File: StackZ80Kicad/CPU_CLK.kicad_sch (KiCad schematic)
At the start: 13 parts, among them SW4 SW_Push, U3 Z84C0008P, U6 74HCT04, Y1 7.3728MHz Crystal

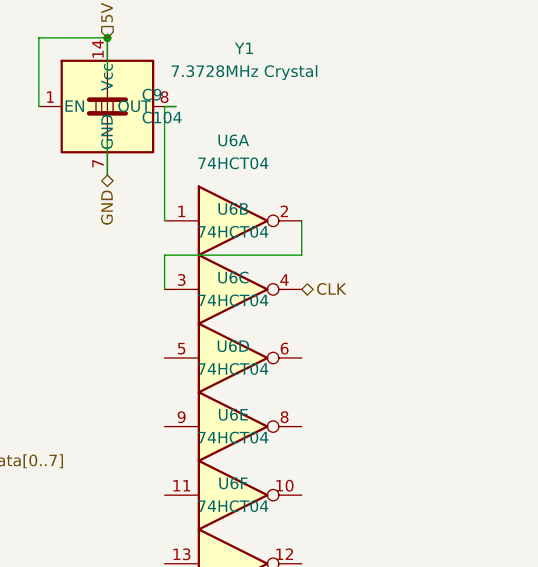
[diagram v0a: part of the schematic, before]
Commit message: Add files via upload
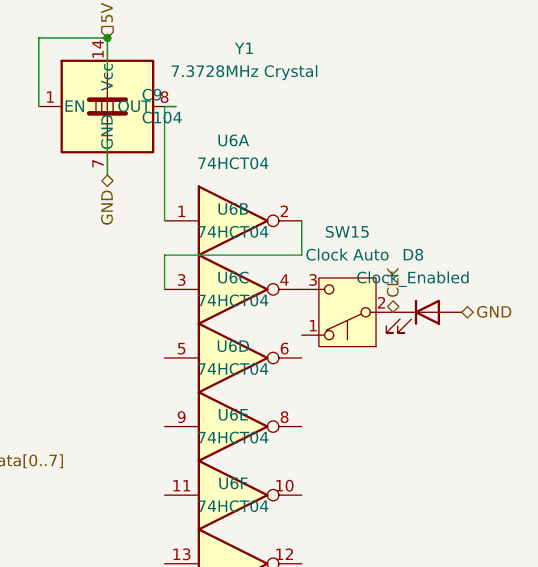
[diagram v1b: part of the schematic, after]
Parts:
- added D8: Clock_Enabled, symbol Device:LED
- added SW15: Clock Auto, symbol Switch:SW_Push_SPDT
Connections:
- net CLK: now also D8.1 (K), SW15.2 (B); no longer U6.4
- net GND: now also D8.2 (A)
- new net: SW15.3 (C), U6.4
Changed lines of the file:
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@@
+		)
+	)
+	(hierarchical_label "GND"
+		(shape bidirectional)
+		(at 137.16 57.15 0)
+		(effects
+			(font
+				(size 1.27 1.27)
+			)
+			(justify left)
 		)
 	)
@@
 		)
 	)
+	(hierarchical_label "CLK"
+		(shape bidirectional)
+		(at 129.54 57.15 90)
+		(effects
+			(font
+				(size 1.27 1.27)
+			)
+			(justify left)
+		)
+	)
 	(hierarchical_label "~{BUSREQ}"
 		(shape bidirectional)
@@
 			)
 			(justify right)
-		)
-	)
-	(hierarchical_label "CLK"
-		(shape bidirectional)
-		(at 119.38 54.61 0)
-		(effects
-			(font
-				(size 1.27 1.27)
-			)
-			(justify left)
 		)
 	)
@@
 	)
 	(symbol
+		(lib_id "Switch:SW_Push_SPDT")
+		(at 124.46 57.15 180)
+		(unit 1)
+		(body_style 1)
+		(exclude_from_sim no)
+		(in_bom yes)
+		(on_board yes)
+		(in_pos_files yes)
+		(dnp no)
+		(fields_autoplaced yes)
+		(property "Reference" "SW15"
+			(at 124.46 48.26 0)
+			(show_name no)
+			(do_not_autoplace no)
+			(effects
+				(font
+					(size 1.27 1.27)
+				)
+			)
+		)
+		(property "Value" "Clock Auto"
+			(at 124.46 50.8 0)
+			(show_name no)
+			(do_not_autoplace no)
+			(effects
+				(font
+					(size 1.27 1.27)
+				)
+			)
+		)
+		(property "Footprint" ""
+			(at 124.46 57.15 0)
+			(hide yes)
+			(show_name no)
+			(do_not_autoplace no)
+			(effects
+				(font
+					(size 1.27 1.27)
+				)
+			)
+		)
+		(property "Datasheet" ""
+			(at 124.46 57.15 0)
+			(hide yes)
+			(show_name no)
+			(do_not_autoplace no)
+			(effects
+				(font
+					(size 1.27 1.27)
+				)
+			)
+		)
+		(property "Description" "Momentary Switch, single pole double throw"
+			(at 124.46 57.15 0)
+			(hide yes)
+			(show_name no)
+			(do_not_autoplace no)
+			(effects
+				(font
+					(size 1.27 1.27)
+				)
+			)
+		)
+		(pin "3"
+		)
+		(pin "2"
+		)
+		(pin "1"
+		)
+		(instances
+			(project "StackZ80Kicad"
+				(path "/4c0a47eb-fb3e-465f-943c-b46f6cbe080d/79d6ed91-38b6-470a-8bf7-3a6bbdac8d22"
+					(reference "SW15")
+					(unit 1)
+				)
+			)
+		)
+	)
+	(symbol
 		(lib_id "Device:R")
 		(at 36.83 76.2 90)
@@
 					(unit 1)
 				)
+			)
+		)
+	)
+	(symbol
+		(lib_id "Device:LED")
+		(at 133.35 57.15 0)
+		(unit 1)
+		(body_style 1)
+		(exclude_from_sim no)
+		(in_bom yes)
+		(on_board yes)
+		(in_pos_files yes)
+		(dnp no)
+		(fields_autoplaced yes)
+		(property "Reference" "D8"
+			(at 131.7625 50.8 0)
+			(show_name no)
+			(do_not_autoplace no)
+			(effects
+				(font
+					(size 1.27 1.27)
+				)
+			)
+		)
+		(property "Value" "Clock_Enabled"
+			(at 131.7625 53.34 0)
+			(show_name no)
+			(do_not_autoplace no)
+			(effects
+				(font
+					(size 1.27 1.27)
+				)
+			)
+		)
+		(property "Footprint" ""
+			(at 133.35 57.15 0)
+			(hide yes)
+			(show_name no)
+			(do_not_autoplace no)
+			(effects
+				(font
+					(size 1.27 1.27)
+				)
+			)
+		)
+		(property "Datasheet" ""
+			(at 133.35 57.15 0)
+			(hide yes)
+			(show_name no)
+			(do_not_autoplace no)
+			(effects
+				(font
+					(size 1.27 1.27)
+				)
+			)
+		)
+		(property "Description" "Light emitting diode"
+			(at 133.35 57.15 0)
+			(hide yes)
+			(show_name no)
+			(do_not_autoplace no)
+			(effects
+				(font
+					(size 1.27 1.27)
+				)
+			)
+		)
+		(property "Sim.Pins" "1=K 2=A"
+			(at 133.35 57.15 0)
+			(hide yes)
+			(show_name no)
+			(do_not_autoplace no)
+			(effects
+				(font
+					(size 1.27 1.27)
+				)
+			)
+		)
+		(pin "2"
+		)
+		(pin "1"
+		)
+		(instances
+			(project "StackZ80Kicad"
+				(path "/4c0a47eb-fb3e-465f-943c-b46f6cbe080d/79d6ed91-38b6-470a-8bf7-3a6bbdac8d22"
+					(reference "D8")
+					(unit 1)
+				)

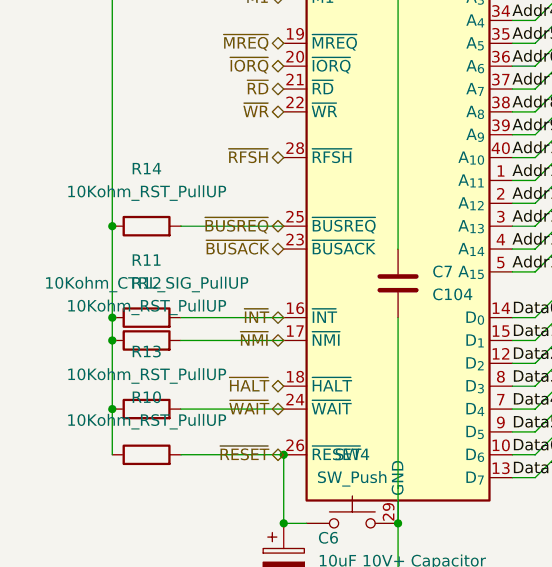
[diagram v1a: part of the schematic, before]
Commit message: Add files via upload
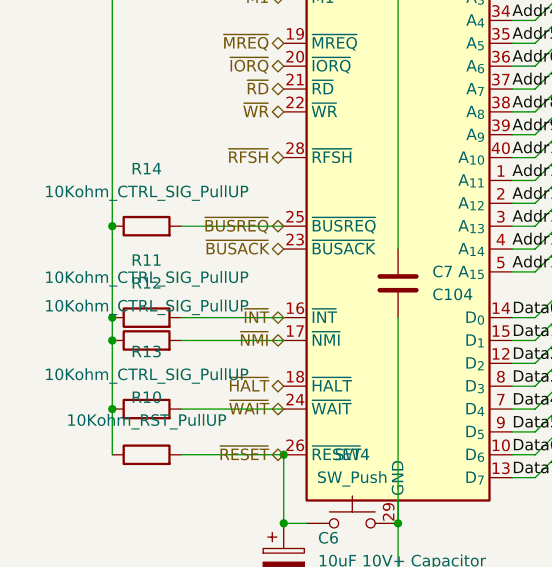
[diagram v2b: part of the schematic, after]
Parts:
- R12, R13, R14: value 10Kohm_RST_PullUP -> 10Kohm_CTRL_SIG_PullUP
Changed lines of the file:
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@@
 		(in_pos_files yes)
 		(dnp no)
-		(fields_autoplaced yes)
 		(property "Reference" "R11"
 			(at 36.83 69.85 90)
@@
 		)
 		(property "Value" "10Kohm_CTRL_SIG_PullUP"
-			(at 36.83 72.39 90)
+			(at 36.83 71.755 90)
 			(show_name no)
 			(do_not_autoplace no)
@@
 			)
 		)
-		(property "Value" "10Kohm_RST_PullUP"
+		(property "Value" "10Kohm_CTRL_SIG_PullUP"
 			(at 36.83 82.55 90)
 			(show_name no)
@@
 			)
 		)
-		(property "Value" "10Kohm_RST_PullUP"
+		(property "Value" "10Kohm_CTRL_SIG_PullUP"
 			(at 36.83 62.23 90)
 			(show_name no)
@@
 			)
 		)
-		(property "Value" "10Kohm_RST_PullUP"
+		(property "Value" "10Kohm_CTRL_SIG_PullUP"
 			(at 36.83 74.93 90)
 			(show_name no)
